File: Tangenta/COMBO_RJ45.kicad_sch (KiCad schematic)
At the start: 1 part, among them J14 RC01133

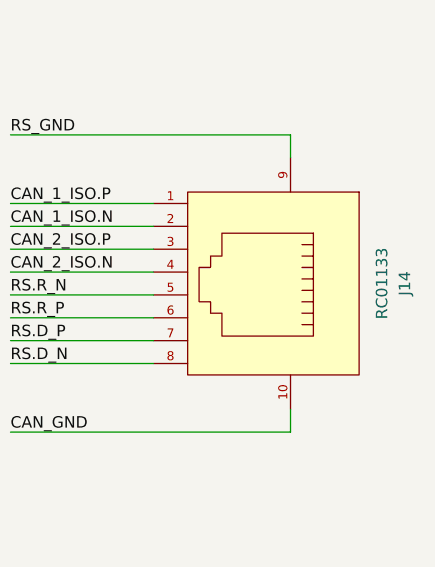
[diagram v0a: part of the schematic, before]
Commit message: initialize branch
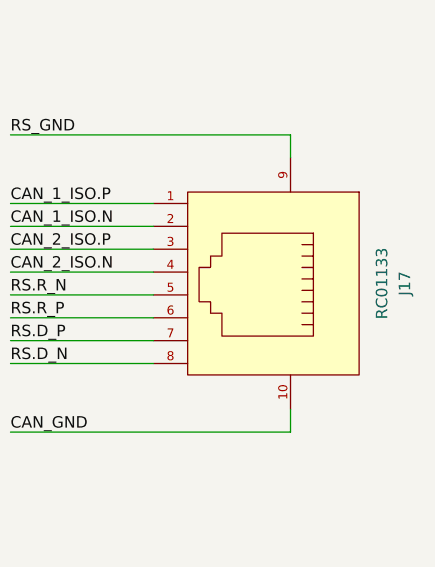
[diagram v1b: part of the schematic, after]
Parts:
- renumbered J14 to J17
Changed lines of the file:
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@@
   (symbol (lib_id "CholaSymbolsPrjLib:RC01133") (at 167.64 97.155 270) (unit 1)
     (in_bom yes) (on_board yes) (dnp no) (fields_autoplaced)
-    (property "Reference" "J14" (at 185.42 95.885 0)
+    (property "Reference" "J17" (at 185.42 95.885 0)
       (effects (font (size 1.27 1.27)))
     )
@@
     (instances
       (project "Tangenta"
-        (path "/358d1bcf-7599-4352-8c4d-baa18a5f09e6/98e3b24f-9927-4339-b8fd-9deea91a522a"
-          (reference "J14") (unit 1)
-        )
         (path "/358d1bcf-7599-4352-8c4d-baa18a5f09e6/da6cda23-cac5-483b-bd71-d8f2b2c13669"
           (reference "J17") (unit 1)

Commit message: J17,U24-26
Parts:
- J17: footprint RJ45_SIMPLE:RJ45_SIMPLE -> CholaFootprintsPrjLib:RJ45_SIMPLE
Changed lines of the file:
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@@
       (effects (font (size 1.27 1.27)))
     )
-    (property "Footprint" "RJ45_SIMPLE:RJ45_SIMPLE" (at 142.24 98.425 0)
+    (property "Footprint" "CholaFootprintsPrjLib:RJ45_SIMPLE" (at 142.24 98.425 0)
       (effects (font (size 1.27 1.27) italic) hide)
     )
